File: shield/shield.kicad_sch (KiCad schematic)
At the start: 12 parts, among them J1 Booster, J2 Battery, P1 Digital, P2 COM, P3 ADC, P4 Analog, P5 ADC, U1 RFM69HW

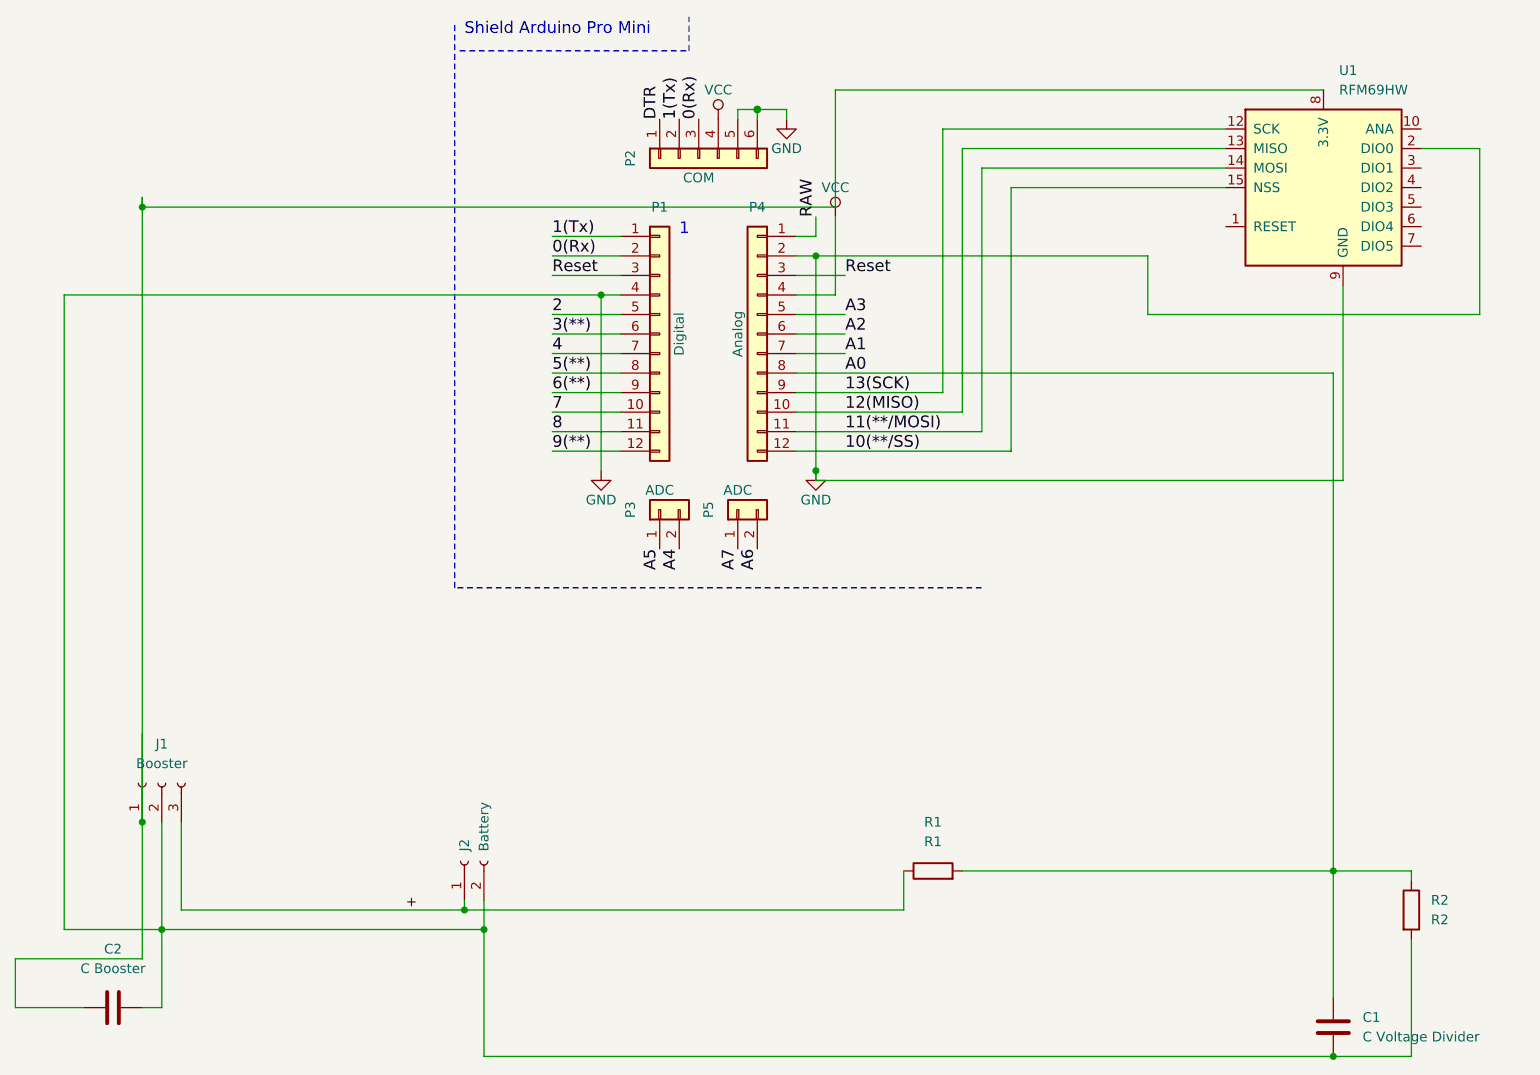
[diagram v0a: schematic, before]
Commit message: pre holiday commit
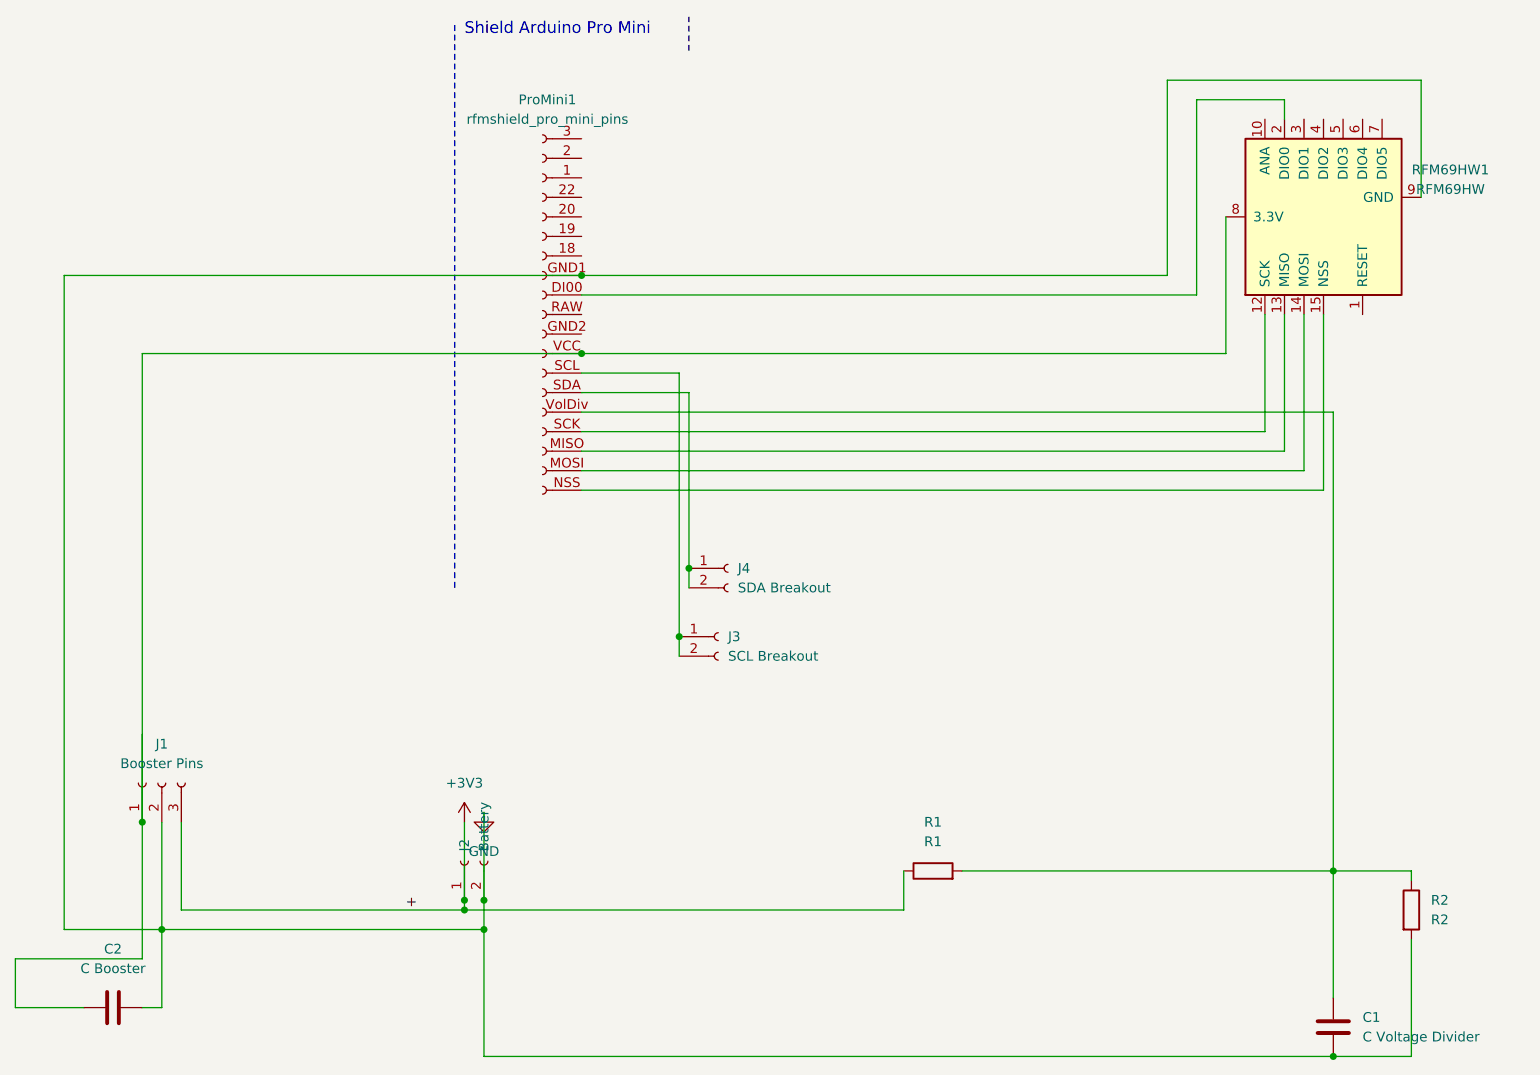
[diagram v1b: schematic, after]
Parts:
- removed P1: Digital, Socket_Arduino_Pro_Mini:Socket_Strip_Arduino_1x12, symbol Connector_Generic:Conn_01x12
- removed P2: COM, Socket_Arduino_Pro_Mini:Socket_Strip_Arduino_1x06, symbol Connector_Generic:Conn_01x06
- removed P3, P5: ADC, Socket_Arduino_Pro_Mini:Socket_Strip_Arduino_1x02, symbol Connector_Generic:Conn_01x02
- removed P4: Analog, Socket_Arduino_Pro_Mini:Socket_Strip_Arduino_1x12, symbol Connector_Generic:Conn_01x12
- removed U1: RFM69HW, RF_Module:HOPERF_RFM69HW, symbol RF_Module:RFM69HW
- added J3: SCL Breakout, Connector_PinHeader_2.54mm:PinHeader_1x02_P2.54mm_Vertical, symbol Connector:Conn_01x02_Female
- added J4: SDA Breakout, Connector_PinHeader_2.54mm:PinHeader_1x02_P2.54mm_Vertical, symbol Connector:Conn_01x02_Female
- added ProMini1: rfmshield_pro_mini_pins, footprints:pro_mini_rfmshield, symbol MySymbols:rfmshield_pro_mini_pins
- added RFM69HW1: RFM69HW, RF_Module:HOPERF_RFM69HW, symbol RF_Module:RFM69HW
- C1, C2: footprint Capacitor_THT:C_Rect_L7.0mm_W3.5mm_P2.50mm_P5.00mm -> Capacitor_THT:CP_Radial_D6.3mm_P2.50mm
- J1: value Booster -> Booster Pins; footprint Connector_PinHeader_2.54mm:PinHeader_1x02_P2.54mm_Horizontal -> Connector_PinHeader_2.54mm:PinHeader_1x03_P2.54mm_Vertical
- J2: footprint Connector_PinHeader_2.54mm:PinHeader_1x03_P2.54mm_Horizontal -> Connector_PinHeader_2.54mm:PinHeader_1x02_P2.54mm_Vertical
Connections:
- net GND: now also ProMini1.GND1, RFM69HW1.11 (GND), RFM69HW1.9 (GND)
- net at C2.1, J1.1 (Pin_1): now also ProMini1.VCC, RFM69HW1.8 (3.3V)
- net + renamed +3V3
- net A0: no longer names the net of C1.1, R1.2, R2.1
- net A0: now also ProMini1.VolDiv
- new net: ProMini1.DI00, RFM69HW1.2 (DIO0)
- new net: ProMini1.MISO, RFM69HW1.13 (MISO)
- new net: ProMini1.MOSI, RFM69HW1.14 (MOSI)
- new net: ProMini1.NSS, RFM69HW1.15 (NSS)
- new net: ProMini1.SCK, RFM69HW1.12 (SCK)
- new net: J3.1 (Pin_1), J3.2 (Pin_2), ProMini1.SCL
- new net: J4.1 (Pin_1), J4.2 (Pin_2), ProMini1.SDA
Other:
- note removed: "1"
